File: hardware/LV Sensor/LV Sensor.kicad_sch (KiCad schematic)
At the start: 68 parts, among them J1 Conn_01x04_Pin, J2 Conn_01x02_Pin, J3 TH, J4 SCREW, J5 TH, J6 SCREW, J7 Conn_01x02_Pin, J8 PWM signal connectors, SW1 SW_Push, U1 MSPM0G3507 RHB32, U10 DXTN80100CFGQ, U2 ISO1042BDW, U3 KA78M05_TO252, U4 KA78M05_TO252, U5 L78L33_SO8, U6 LMV324, U7 HBDM60V600X, U9 DXTN80100CFGQ

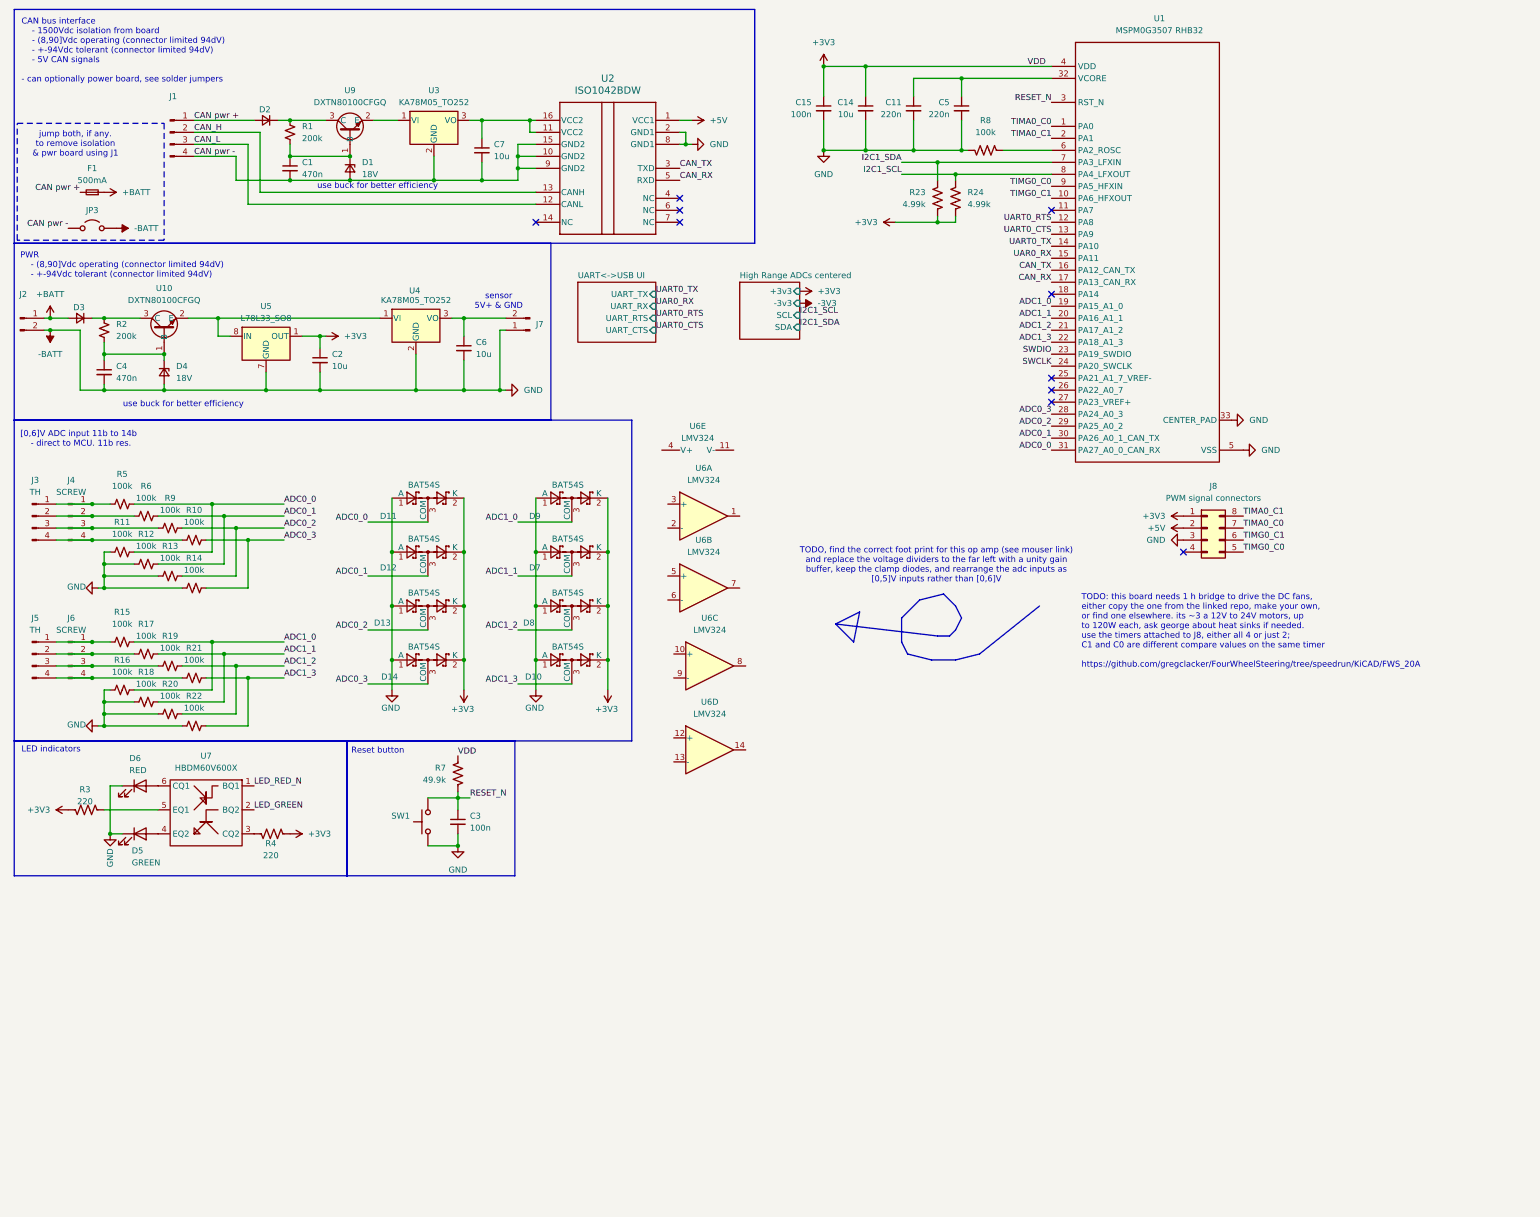
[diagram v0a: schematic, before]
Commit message: bluhhh
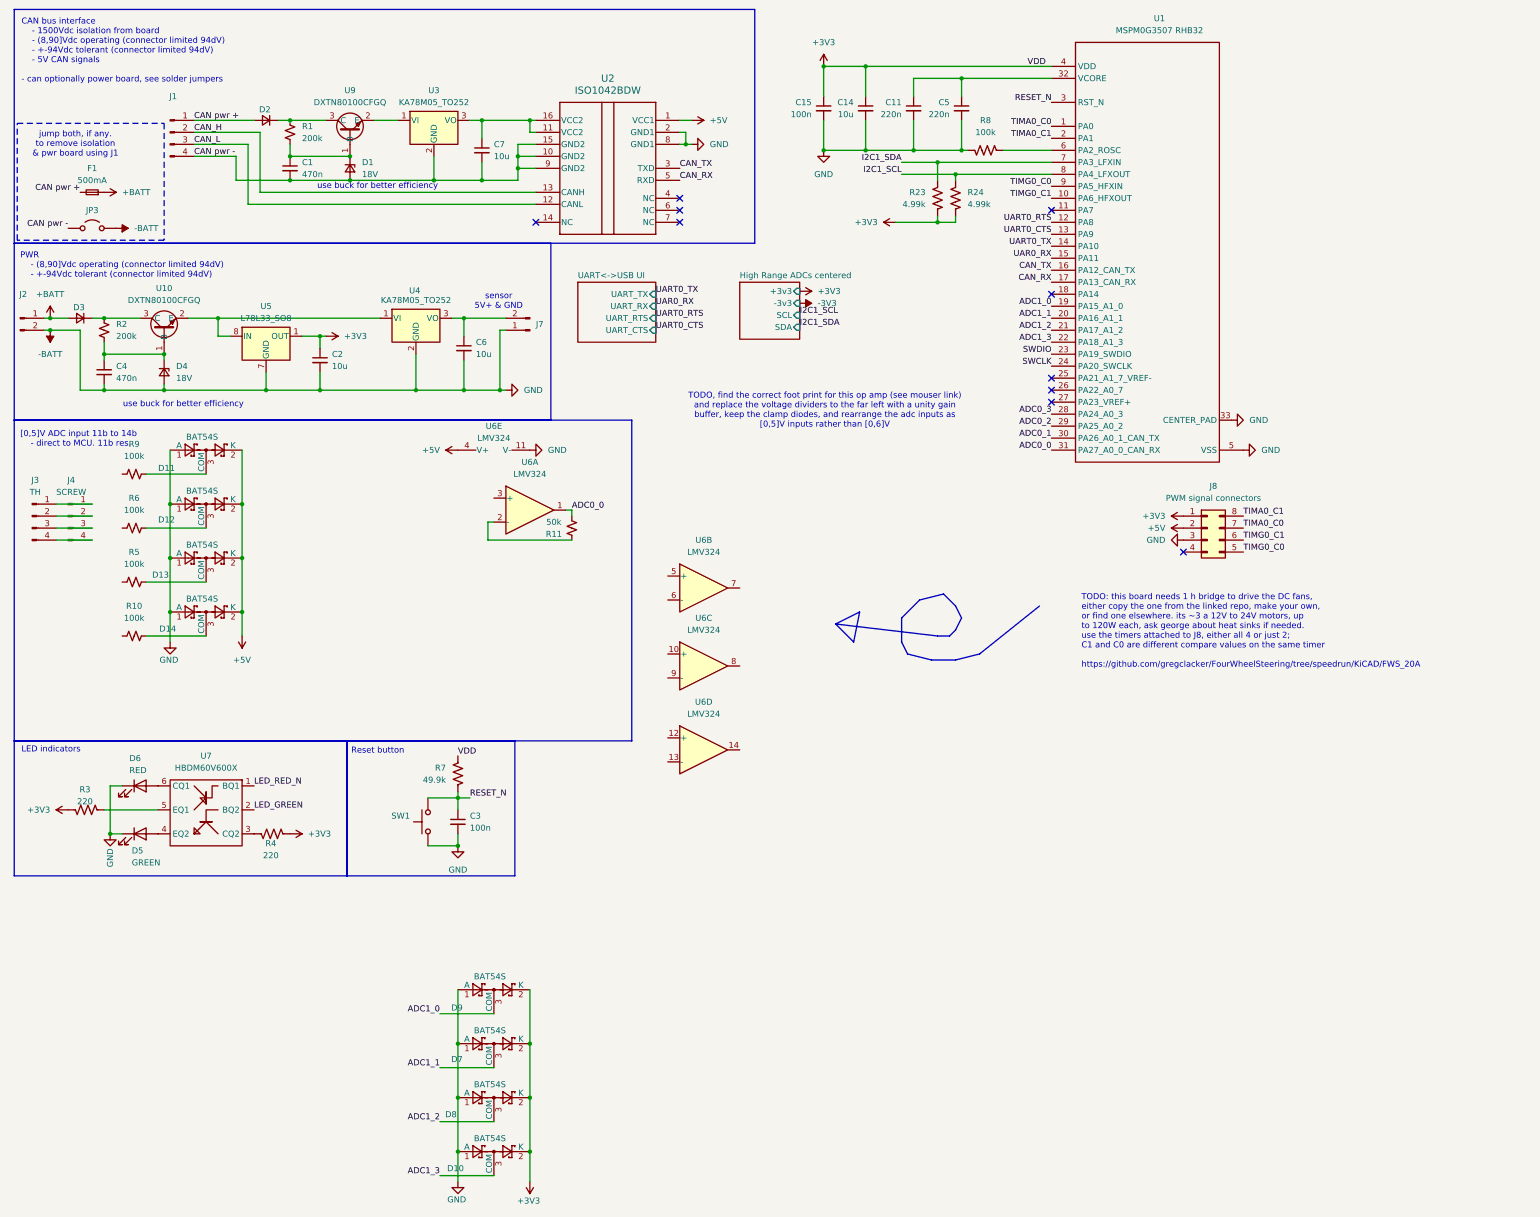
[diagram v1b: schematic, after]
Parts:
- removed J5: TH, Connector_PinHeader_2.54mm:PinHeader_1x04_P2.54mm_Vertical, symbol Connector:Conn_01x04_Pin
- removed J6: SCREW, TerminalBlock:TerminalBlock_MaiXu_MX126-5.0-04P_1x04_P5.00mm, symbol Connector:Conn_01x04_Pin
- removed R12, R13, R14, R15, R16, R17, R18, R19, R20, R21, R22: 100k, symbol Device:R_Small_US
- R10, R5, R6, R9: footprint (none) -> Resistor_SMD:R_1206_3216Metric_Pad1.30x1.75mm_HandSolder
- R11: value 100k -> 50k; footprint (none) -> Resistor_SMD:R_1206_3216Metric_Pad1.30x1.75mm_HandSolder; mouser https://www.mouser.com/ProductDetail/YAGEO/RC1206FR-07100KL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 -> https://www.mouser.com/ProductDetail/YAGEO/RT1206BRD0750KL?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; unit x1 0.10 -> 0.21; unit x10 0.016 -> 0.161
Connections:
- net +3V3: no longer D11.2 (K), D12.2 (K), D13.2 (K), D14.2 (K)
- net +5V: now also D11.2 (K), D12.2 (K), D13.2 (K), D14.2 (K), U6.4 (V+)
- net -BATT: now also U6.11 (V-); no longer R11.1
- net ADC0_0: now also U6.1; no longer D11.3 (COM), R5.2
- net ADC0_1: no longer D12.3 (COM), R6.2
- net ADC0_2: no longer D13.3 (COM), R9.2
- net ADC0_3: no longer D14.3 (COM), R10.2
- net at J3.3 (Pin_3), J4.3 (Pin_3): no longer R9.1
- net at J3.2 (Pin_2), J4.2 (Pin_2): no longer R6.1
- net at J3.4 (Pin_4), J4.4 (Pin_4): no longer R10.1
- net at J3.1 (Pin_1), J4.1 (Pin_1): no longer R5.1
- net at U6.2 (-): now also R11.1
- new net: D11.3 (COM), R9.2
- new net: D13.3 (COM), R5.2
- new net: D14.3 (COM), R10.2
- new net: D12.3 (COM), R6.2
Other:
- note added: "[0,5]V ADC input 11b to 14b - direct to MCU. 11b res."
- note removed: "[0,6]V ADC input 11b to 14b - direct to MCU. 11b res."
- moved on the sheet: D10, D11, D12, D13, D14, D7, D8, D9, R10, U6A, U6C, U6D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
